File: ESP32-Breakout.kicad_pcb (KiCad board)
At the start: 2 copper layers, 44.5 x 49.5 mm, 3 parts, among them J101 Conn_01x19, J102 Conn_01x19, U101 ESP32-DEVKITC-32D

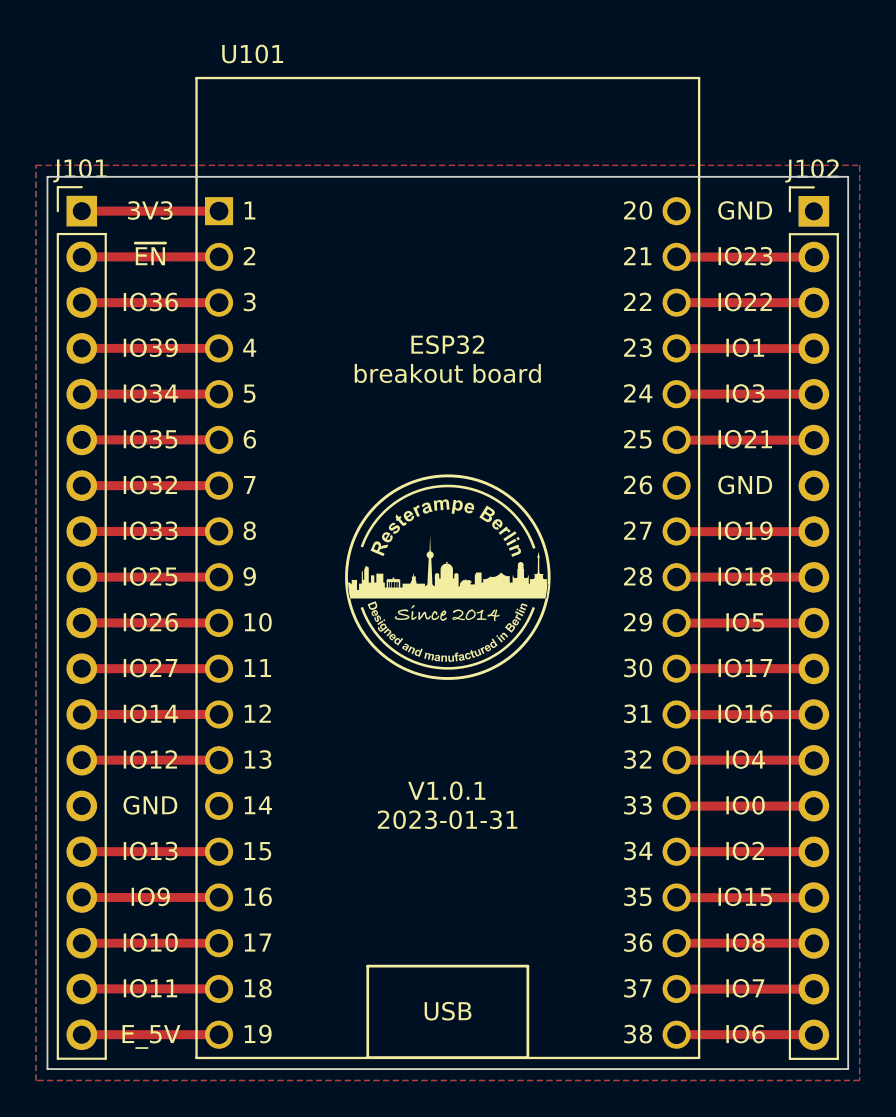
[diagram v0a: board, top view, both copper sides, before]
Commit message: Closed #1
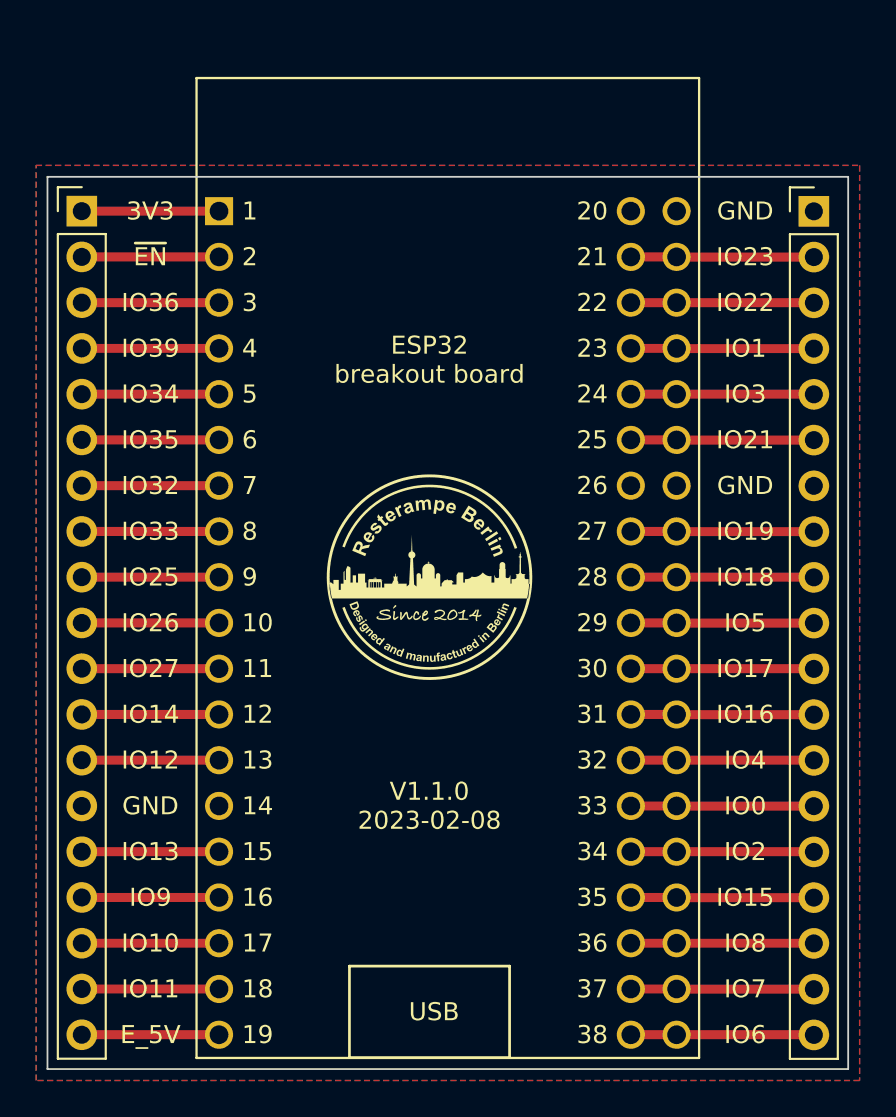
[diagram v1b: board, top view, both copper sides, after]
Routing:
- net Net-(J102-Pad8): track 7.62 -> 10.2 mm
- net Net-(J102-Pad6): track 7.62 -> 10.2 mm
- net Net-(J102-Pad5): track 7.62 -> 10.2 mm
- net Net-(J102-Pad4): track 7.62 -> 10.2 mm
- net Net-(J102-Pad3): track 7.62 -> 10.2 mm
- net Net-(J102-Pad19): track 7.62 -> 10.2 mm
- net Net-(J102-Pad17): track 7.62 -> 10.2 mm
- net Net-(J102-Pad15): track 7.62 -> 10.2 mm
- net Net-(J102-Pad13): track 7.62 -> 10.2 mm
- net Net-(J102-Pad12): track 7.62 -> 10.2 mm
- net Net-(J102-Pad10): track 7.62 -> 10.2 mm
- net Net-(J102-Pad9): track 7.62 -> 10.2 mm
- net Net-(J102-Pad2): track 7.62 -> 10.2 mm
- net Net-(J102-Pad18): track 7.62 -> 10.2 mm
- net Net-(J102-Pad16): track 7.62 -> 10.2 mm
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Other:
- board text added: "This is the smaller 32S board (fits well on breadboard)"
- board text added: "This is the wider 32D board"
